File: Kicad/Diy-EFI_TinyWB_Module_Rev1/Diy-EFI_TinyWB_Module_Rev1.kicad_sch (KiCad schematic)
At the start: 1 part, among them J1 TinyWB_Conn_01x06_&_01x04_Male

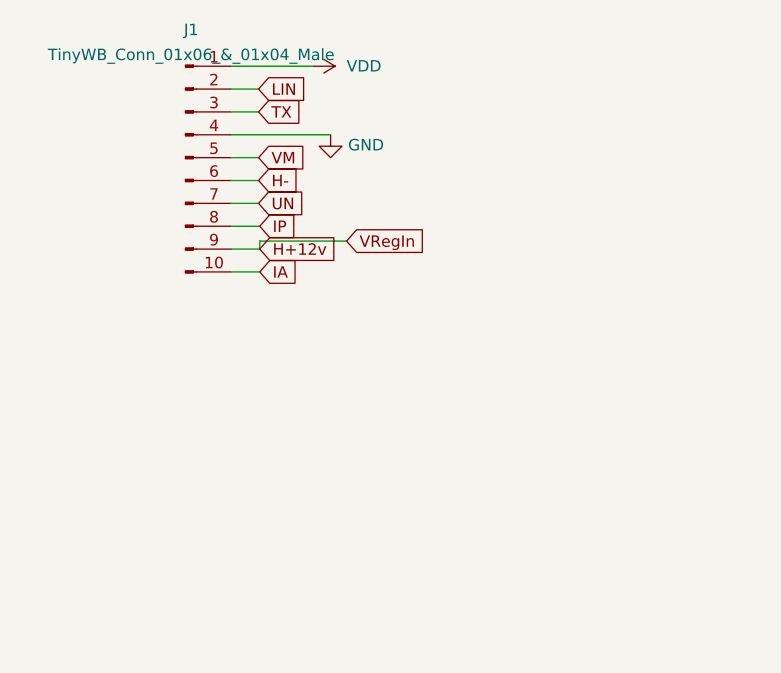
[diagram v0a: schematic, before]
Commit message: maj
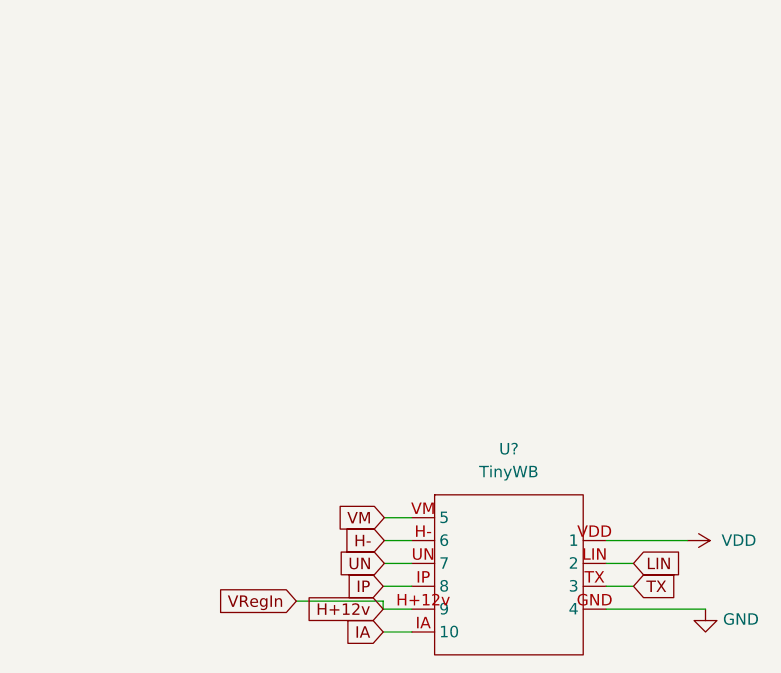
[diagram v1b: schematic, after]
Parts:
- removed J1: TinyWB_Conn_01x06_&_01x04_Male, Connector_PinHeader_2.54mm:PinHeader_1x06_P2.54mm_Vertical, symbol Connector:Conn_01x10_Male
- added U?: TinyWB, symbol AmesisProject_Librairie:TinyWB
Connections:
- net GND: now also U?.GND (4)
- net H+12v: now also U?.H+12v (9)
- net H-: now also U?.H- (6)
- net IA: now also U?.IA (10)
- net IP: now also U?.IP (8)
- net LIN: now also U?.LIN (2)
- net TX: now also U?.TX (3)
- net UN: now also U?.UN (7)
- net VDD: now also U?.VDD (1)
- net VM: now also U?.VM (5)
